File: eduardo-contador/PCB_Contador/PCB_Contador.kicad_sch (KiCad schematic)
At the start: 57 parts, among them J1 Screw_Terminal_01x02, SW1 SW_DIP_x04, SW3 SW_DIP_x04, SW4 SW_DIP_x04, U1 74LS47, U2 74LS190, U3 74LS47, U4 74LS190, U5 74LS190, U6 74LS47, U7 LM555xN

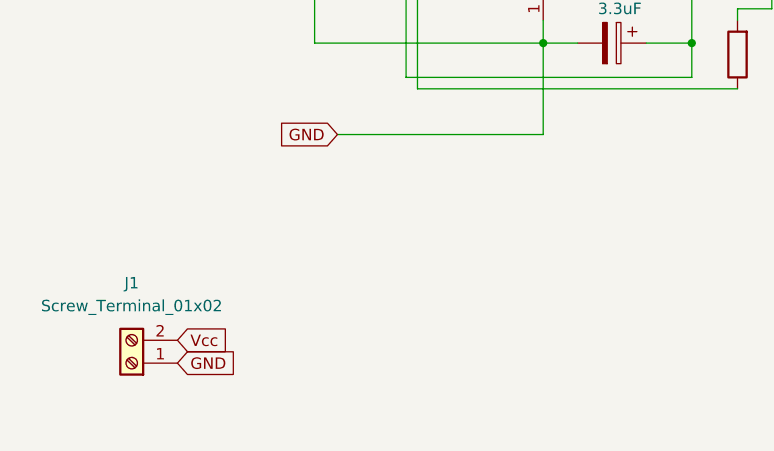
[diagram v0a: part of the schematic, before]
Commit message: cambios eduardo
Actualizacion
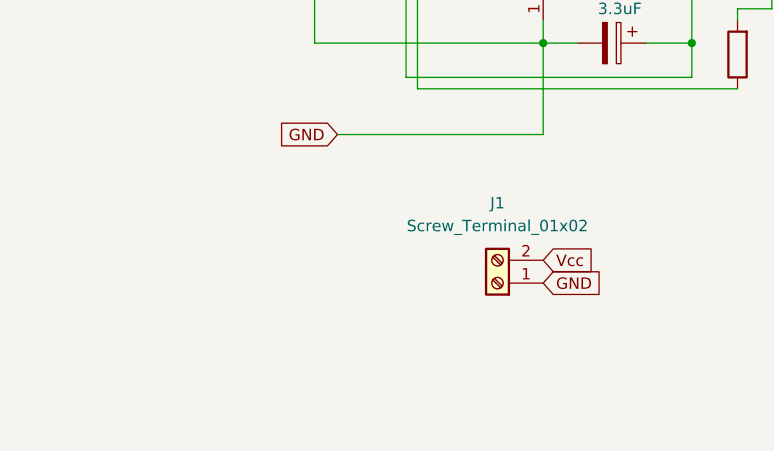
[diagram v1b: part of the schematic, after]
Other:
- moved on the sheet: J1
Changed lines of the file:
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@@
 	(global_label "GND"
 		(shape input)
-		(at 64.77 148.59 0)
+		(at 105.41 139.7 0)
 		(fields_autoplaced yes)
 		(effects
@@
 		)
 		(property "Intersheetrefs" "${INTERSHEET_REFS}"
-			(at 71.6257 148.59 0)
+			(at 112.2657 139.7 0)
 			(effects
 				(font
@@
 	(global_label "Vcc"
 		(shape input)
-		(at 64.77 146.05 0)
+		(at 105.41 137.16 0)
 		(fields_autoplaced yes)
 		(effects
@@
 		)
 		(property "Intersheetrefs" "${INTERSHEET_REFS}"
-			(at 71.021 146.05 0)
+			(at 111.661 137.16 0)
 			(effects
 				(font
@@
 	(symbol
 		(lib_id "Connector:Screw_Terminal_01x02")
-		(at 59.69 148.59 180)
+		(at 100.33 139.7 180)
 		(unit 1)
 		(exclude_from_sim no)
@@
 		(fields_autoplaced yes)
 		(property "Reference" "J1"
-			(at 59.69 139.7 0)
+			(at 100.33 130.81 0)
 			(effects
 				(font
@@
 		)
 		(property "Value" "Screw_Terminal_01x02"
-			(at 59.69 142.24 0)
+			(at 100.33 133.35 0)
 			(effects
 				(font
@@
 		)
 		(property "Footprint" "TerminalBlock:TerminalBlock_Xinya_XY308-2.54-2P_1x02_P2.54mm_Horizontal"
-			(at 59.69 148.59 0)
+			(at 100.33 139.7 0)
 			(effects
 				(font
@@
 		)
 		(property "Datasheet" "~"
-			(at 59.69 148.59 0)
+			(at 100.33 139.7 0)
 			(effects
 				(font
@@
 		)
 		(property "Description" "Generic screw terminal, single row, 01x02, script generated (kicad-library-utils/schlib/autogen/connector/)"
-			(at 59.69 148.59 0)
-			(effects
-				(font
+			(at 100.33 139.7 0)
+			(effects
+				(font
